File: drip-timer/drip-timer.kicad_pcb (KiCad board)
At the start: 2 copper layers, 50.5 x 62.7 mm, 12 parts, among them J1 BATT, J2 VALVE, J3 FLASH, J4 Flash TS, K1 DIPxx-1Axx-11x, SW1 GO, U1 ProMicro, U3 MOC3021

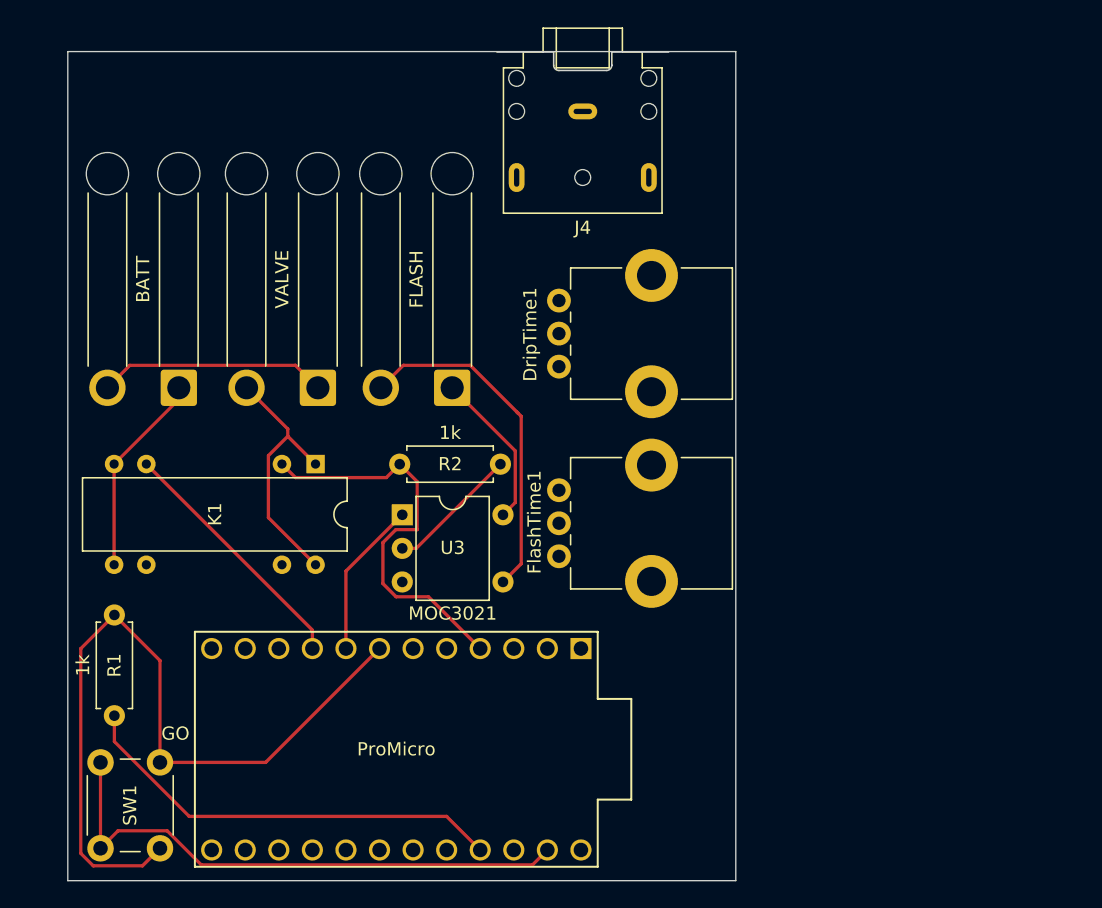
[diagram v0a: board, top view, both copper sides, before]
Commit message: completed work on v0.1 of pcb
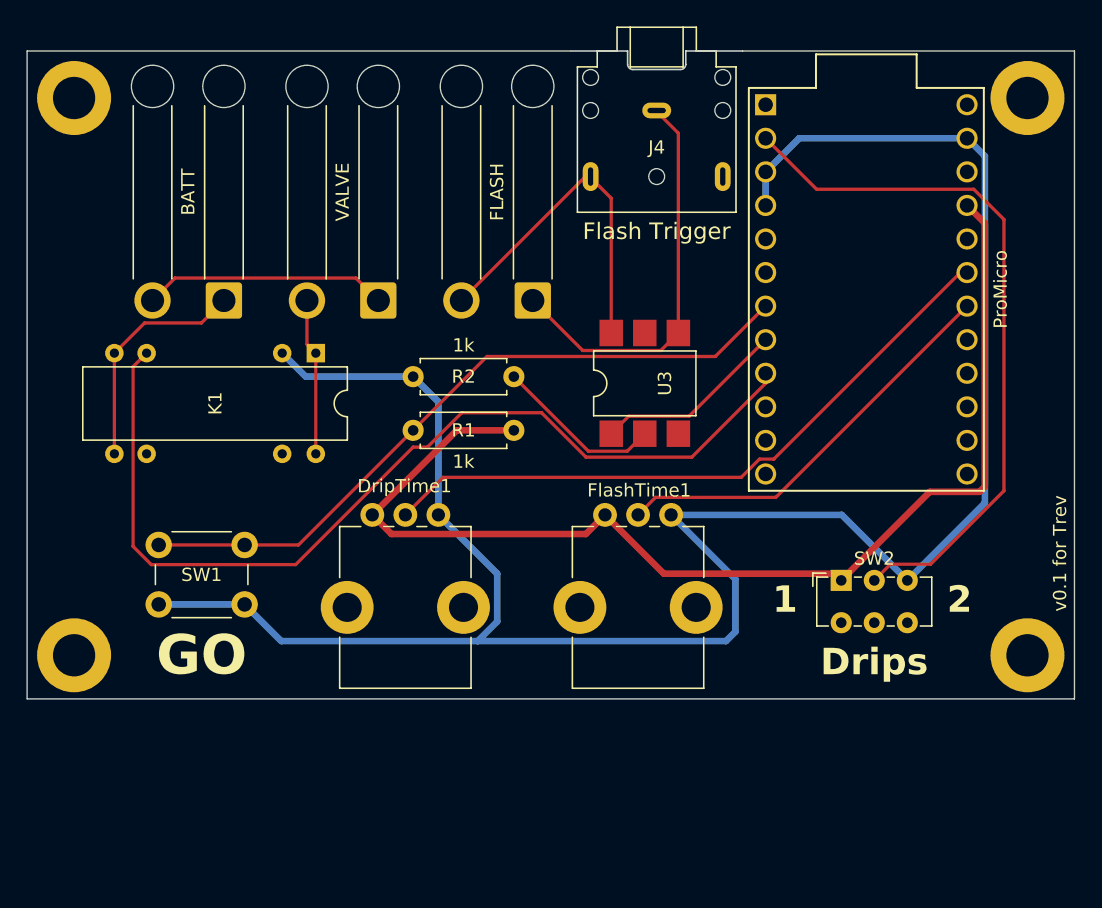
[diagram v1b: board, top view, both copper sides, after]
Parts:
- added REF**: MountingHole_3.2mm_M3_DIN965_Pad, MountingHole:MountingHole_3.2mm_M3_DIN965_Pad, F.Cu at (129.0, 84.3)
- added REF**: MountingHole_3.2mm_M3_DIN965_Pad, MountingHole:MountingHole_3.2mm_M3_DIN965_Pad, F.Cu at (201.2, 42.2)
- added REF**: MountingHole_3.2mm_M3_DIN965_Pad, MountingHole:MountingHole_3.2mm_M3_DIN965_Pad, F.Cu at (129.0, 42.2)
- added REF**: MountingHole_3.2mm_M3_DIN965_Pad, MountingHole:MountingHole_3.2mm_M3_DIN965_Pad, F.Cu at (201.2, 84.3)
- added SW2: Drips, Button_Switch_THT:SW_E-Switch_EG1271_SPDT, F.Cu at (187.1, 78.7)
- DripTime1, FlashTime1: value R_Potentiometer -> 10k
- J4: value Flash TS -> Flash Trigger
- U3: value MOC3021 -> MOC3021S; footprint Package_DIP:Toshiba_11-7A9 -> Package_DIP:SMDIP-6_W7.62mm
- moved U1 49.8 mm to (189.0, 56.6), turned to -90 degrees
- moved R1 26.6 mm to (154.7, 67.3), turned to 0 degrees
- moved SW1 21.4 mm to (141.9, 80.5), turned to 180 degrees
- moved U3 20.9 mm to (172.2, 63.8), turned to 90 degrees
- moved DripTime1 18.0 mm to (151.6, 73.7), turned to -90 degrees
- moved J3 8.99 mm to (163.7, 57.5)
- moved K1 8.39 mm to (147.3, 61.5)
- moved J2 8.03 mm to (152.1, 57.5)
- moved J1 7.43 mm to (140.4, 57.5)
- moved R2 6.70 mm to (162.3, 63.2)
- moved J4 5.60 mm to (173.1, 43.1)
- moved FlashTime1 4.69 mm to (169.2, 73.7), turned to -90 degrees
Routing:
- net GND: track 73.1 -> 165.0 mm
- net VCC: track 33.0 -> 87.7 mm
- net Net-(SW2-B): track 0.00 -> 53.7 mm
- net Net-(U1-D7): track 19.2 -> 72.7 mm
- net Net-(U1-F5): track 0.00 -> 50.1 mm
- net Net-(U1-F6): track 0.00 -> 31.4 mm
- net Net-(J3-Pin_1): track 12.0 -> 30.6 mm
- net Net-(J2-Pin_2): track 19.7 -> 11.9 mm
- net Net-(U1-D4): track 58.8 -> 53.4 mm
- net Net-(U1-C6): track 11.9 -> 14.6 mm
- net Net-(R2-Pad1): track 10.1 -> 12.8 mm
- net Net-(J1-Pin_1): track 15.4 -> 17.6 mm
- net Net-(J1-Pin_2): track 17.3 -> 18.5 mm
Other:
- board size 50.5 x 62.7 mm -> 79.2 x 49 mm
- board text added: "1"
- board text added: "2"
- board text added: "v0.1 for Trev"
